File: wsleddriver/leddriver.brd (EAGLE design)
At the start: 29.9 x 14.3 mm, 17 parts, among them IC1 WS2811-SOP8

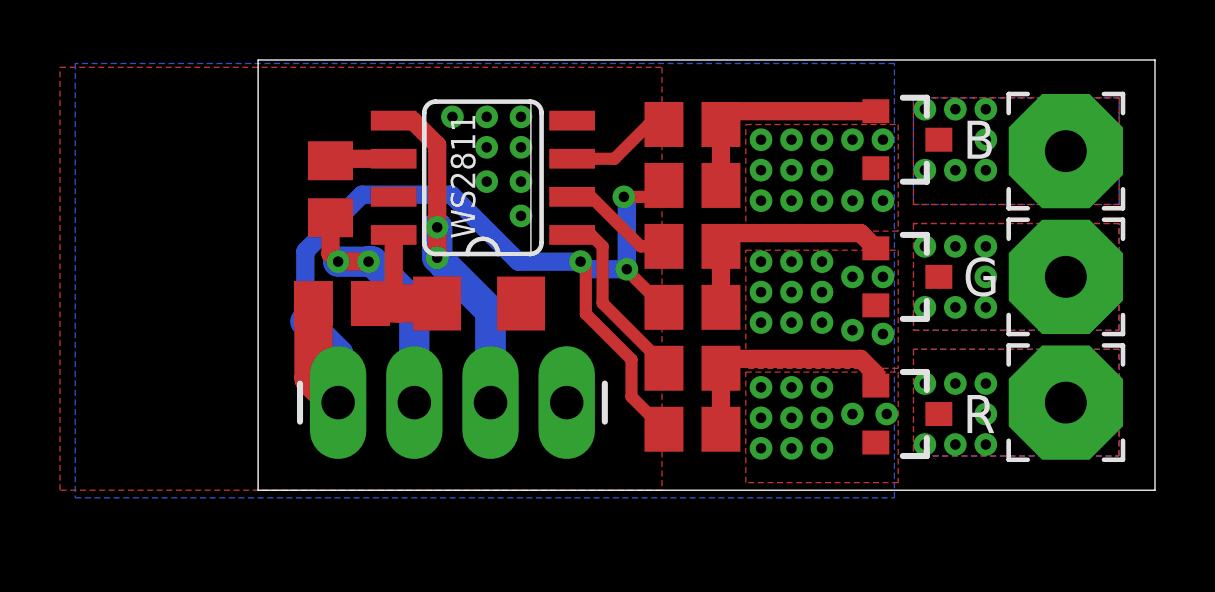
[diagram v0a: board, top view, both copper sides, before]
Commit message: c
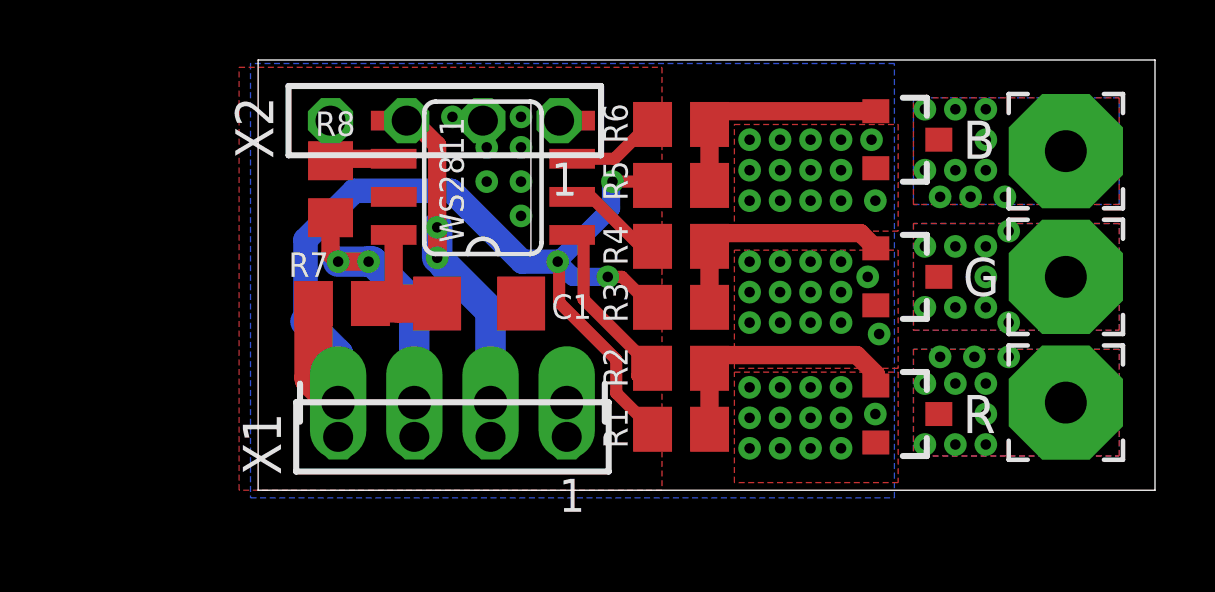
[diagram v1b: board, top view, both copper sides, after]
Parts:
- removed R10: 100, rcl:R0805
- removed R9: 10k, rcl:R0805
- added R1: 10k, rcl:R0805
- added R2: 100, rcl:R0805
- added X1, X2: TSW-104-07-G-S, con-samtec:TSW-104-XX-G-S
- R4: value 10k -> 100
- R5: value 100 -> 10k
- moved R4 2.07 mm to (19.4, 7.87)
- moved R5 2.07 mm to (19.4, 9.91)
- moved R3 0.38 mm to (19.4, 5.84)
- moved R6 0.38 mm to (19.4, 11.9)
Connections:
- net +12V: now also R1.1, R5.1; no longer R4.1, R9.1
- net G: now also R4.1; no longer R5.1
- net N$2: now also R4.2; no longer R5.2
- net N$3: now also R5.2; no longer R4.2
- net N$4: now also R1.2, R2.2; no longer R10.2, R9.2
- net R: now also R2.1; no longer R10.1
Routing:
- net +12V: track 34.1 -> 35.1 mm
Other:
- board text added: "C1"
- board text added: "R1"
- board text added: "R2"
- board text added: "R3"
- board text added: "R4"
- board text added: "R5"
- board text added: "R6"
- board text added: "R7"
- board text added: "R8"

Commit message: w
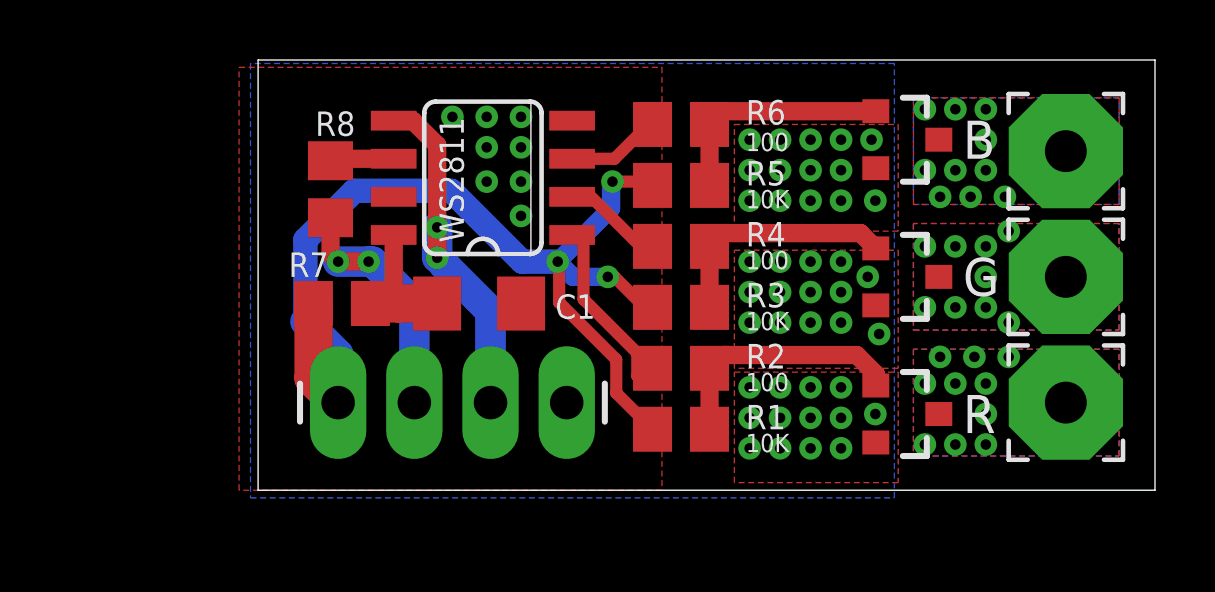
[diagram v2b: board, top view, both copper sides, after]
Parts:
- removed X1, X2: TSW-104-07-G-S, con-samtec:TSW-104-XX-G-S
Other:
- board text added: "100"
- board text added: "10K"
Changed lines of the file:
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@@
 <?xml version="1.0" encoding="utf-8"?>
 <!DOCTYPE eagle SYSTEM "eagle.dtd">
-<eagle version="9.2.2">
+<eagle version="9.4.2">
 <drawing>
 <settings>
@@
 <text x="28.829" y="10.795" size="1.27" layer="25" font="vector" ratio="15">B</text>
 <text x="12.192" y="8.001" size="0.8128" layer="25" font="vector" ratio="15" rot="R90">WS2811</text>
-<text x="17.653" y="1.143" size="0.8128" layer="25" font="vector" ratio="15" rot="R90">R1</text>
-<text x="17.653" y="3.175" size="0.8128" layer="25" font="vector" ratio="15" rot="R90">R2</text>
-<text x="17.653" y="7.239" size="0.8128" layer="25" font="vector" ratio="15" rot="R90">R4</text>
-<text x="17.653" y="9.398" size="0.8128" layer="25" font="vector" ratio="15" rot="R90">R5</text>
-<text x="17.653" y="11.303" size="0.8128" layer="25" font="vector" ratio="15" rot="R90">R6</text>
-<text x="17.653" y="5.334" size="0.8128" layer="25" font="vector" ratio="15" rot="R90">R3</text>
-<text x="15.113" y="5.461" size="0.8128" layer="25" font="vector" ratio="15">C1</text>
+<text x="21.59" y="1.778" size="0.8128" layer="25" font="vector" ratio="15">R1</text>
+<text x="21.59" y="3.81" size="0.8128" layer="25" font="vector" ratio="15">R2</text>
+<text x="21.59" y="7.874" size="0.8128" layer="25" font="vector" ratio="15">R4</text>
+<text x="21.59" y="9.906" size="0.8128" layer="25" font="vector" ratio="15">R5</text>
+<text x="21.59" y="11.938" size="0.8128" layer="25" font="vector" ratio="15">R6</text>
+<text x="21.59" y="5.842" size="0.8128" layer="25" font="vector" ratio="15">R3</text>
+<text x="15.24" y="5.461" size="0.8128" layer="25" font="vector" ratio="15">C1</text>
 <text x="7.239" y="11.557" size="0.8128" layer="25" font="vector" ratio="15">R8</text>
 <text x="6.35" y="6.858" size="0.8128" layer="25" font="vector" ratio="15">R7</text>
+<text x="21.59" y="11.049" size="0.6096" layer="25" font="vector" ratio="15">100</text>
+<text x="21.59" y="9.144" size="0.6096" layer="25" font="vector" ratio="15">10K</text>
+<text x="21.59" y="5.08" size="0.6096" layer="25" font="vector" ratio="15">10K</text>
+<text x="21.59" y="1.016" size="0.6096" layer="25" font="vector" ratio="15">10K</text>
+<text x="21.59" y="7.112" size="0.6096" layer="25" font="vector" ratio="15">100</text>
+<text x="21.59" y="3.048" size="0.6096" layer="25" font="vector" ratio="15">100</text>
 </plain>
 <attributes>
@@
 <attribute name="VALUE" x="32.258" y="12.249" size="0.0254" layer="27"/>
 </element>
-<element name="X1" library="con-samtec" library_urn="urn:adsk.eagle:library:184" package="TSW-104-XX-G-S" value="TSW-104-07-G-S" x="11.811" y="1.524" smashed="yes">
-<attribute name="MF" value="Samtec Inc." x="11.811" y="1.524" size="1.778" layer="27" display="off"/>
-<attribute name="MPN" value="TSW-104-07-G-S" x="11.811" y="1.524" size="1.778" layer="27" display="off"/>
-<attribute name="NAME" x="6.096" y="0.254" size="1.27" layer="25" rot="R90"/>
-<attribute name="OC_FARNELL" value="" x="11.811" y="1.524" size="1.778" layer="27" display="off"/>
-<attribute name="OC_NEWARK" value="" x="11.811" y="1.524" size="1.778" layer="27" display="off"/>
-<attribute name="VALUE" x="18.796" y="0.254" size="1.27" layer="27" rot="R90"/>
-</element>
-<element name="X2" library="con-samtec" library_urn="urn:adsk.eagle:library:184" package="TSW-104-XX-G-S" value="TSW-104-07-G-S" x="11.557" y="12.065" smashed="yes">
-<attribute name="MF" value="Samtec Inc." x="11.557" y="12.065" size="1.778" layer="27" display="off"/>
-<attribute name="MPN" value="TSW-104-07-G-S" x="11.557" y="12.065" size="1.778" layer="27" display="off"/>
-<attribute name="NAME" x="5.842" y="10.795" size="1.27" layer="25" rot="R90"/>
-<attribute name="OC_FARNELL" value="" x="11.557" y="12.065" size="1.778" layer="27" display="off"/>
-<attribute name="OC_NEWARK" value="" x="11.557" y="12.065" size="1.778" layer="27" display="off"/>
-<attribute name="VALUE" x="18.542" y="10.795" size="1.27" layer="27" rot="R90"/>
-</element>
 </elements>
 <signals>
@@
 <contactref element="R3" pad="1"/>
 <contactref element="R5" pad="1"/>
-<wire x1="16.9898" y1="6.858" x2="17.465" y2="6.858" width="0.4064" layer="1"/>
-<wire x1="18.481" y1="5.842" x2="17.465" y2="6.858" width="0.4064" layer="1"/>
+<wire x1="18.227" y1="5.842" x2="17.211" y2="6.858" width="0.4064" layer="1"/>
+<wire x1="16.9898" y1="6.858" x2="17.211" y2="6.858" width="0.4064" layer="1"/>
+<wire x1="18.481" y1="5.842" x2="18.227" y2="5.842" width="0.4064" layer="1"/>
 <via x="16.9898" y="6.858" extent="1-16" drill="0.35"/>
 <wire x1="18.481" y1="9.906" x2="18.354" y2="10.033" width="0.4064" layer="1"/>
